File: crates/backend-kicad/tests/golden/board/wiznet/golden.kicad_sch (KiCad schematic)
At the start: 1 part, among them U1 U

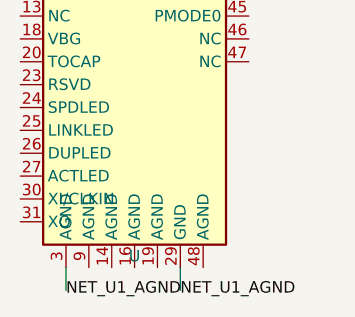
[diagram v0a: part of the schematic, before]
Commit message: Apply stabilise-copperleaf-pipeline
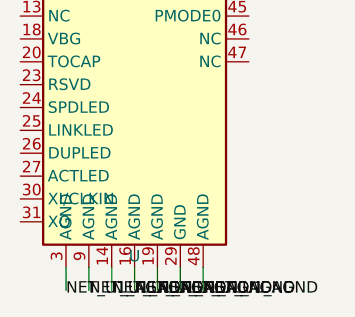
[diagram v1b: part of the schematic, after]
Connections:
- net NET_U1_AGND: now also U1.14 (AGND), U1.16 (AGND), U1.19 (AGND), U1.48 (AGND), U1.9 (AGND)
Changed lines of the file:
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@@
+  (wire
+    (pts
+      (xy 35.56 99.06)
+      (xy 35.56 101.6))
+    (stroke
+      (width 0))
+)
+  (label "NET_U1_AGND"
+    (at 35.56 101.6 0)
+    (effects
+      (font
+        (size 1.27 1.27)))
+)
+  (wire
+    (pts
+      (xy 38.1 99.06)
+      (xy 38.1 101.6))
+    (stroke
+      (width 0))
+)
+  (label "NET_U1_AGND"
+    (at 38.1 101.6 0)
+    (effects
+      (font
+        (size 1.27 1.27)))
+)
+  (wire
+    (pts
+      (xy 40.64 99.06)
+      (xy 40.64 101.6))
+    (stroke
+      (width 0))
+)
+  (label "NET_U1_AGND"
+    (at 40.64 101.6 0)
+    (effects
+      (font
+        (size 1.27 1.27)))
+)
+  (wire
+    (pts
+      (xy 43.18 99.06)
+      (xy 43.18 101.6))
+    (stroke
+      (width 0))
+)
+  (label "NET_U1_AGND"
+    (at 43.18 101.6 0)
+    (effects
+      (font
+        (size 1.27 1.27)))
+)
   (wire
     (pts
@@
     (effects
       (font
+        (size 1.27 1.27)))
+)
+  (wire
+    (pts
+      (xy 48.26 99.06)
+      (xy 48.26 101.6))
+    (stroke
+      (width 0))
+)
+  (label "NET_U1_AGND"
+    (at 48.26 101.6 0)
+    (effects
+      (font
